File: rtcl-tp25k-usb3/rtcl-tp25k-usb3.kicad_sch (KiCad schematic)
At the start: 65 parts, among them J1 ZX360D-B-10P(30), J10 SSQ-106-02-F-D-RA, J2 0525592253, J3 BTB-DF40C-60DS-0.4V(51), J4 DF40C-60DS-0.4V(51), J5 JTAG, U1 FT601Q, U2 TPD4E05U06DQA, U3 USBLC6-2P6, U4 TPS62826DMQR, X1 ABM3-30.000MHZ-D2Y-T

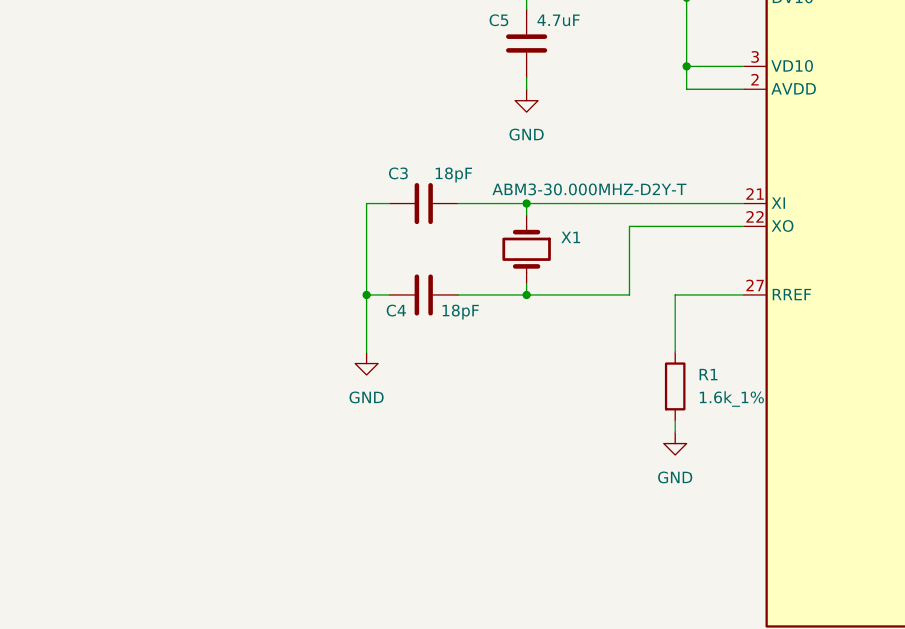
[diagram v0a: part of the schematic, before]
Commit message: WIP
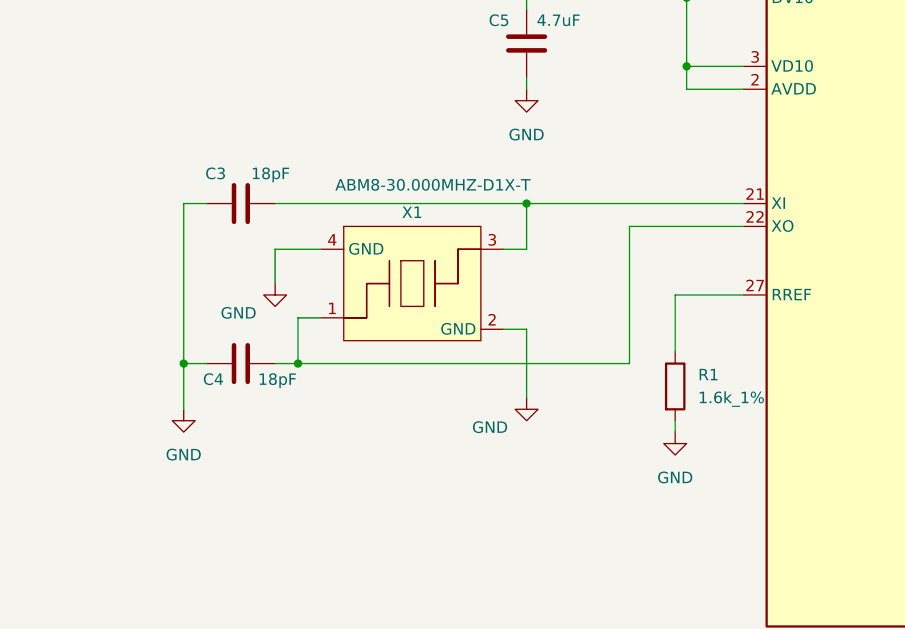
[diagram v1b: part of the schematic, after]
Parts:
- removed X1: ABM3-30.000MHZ-D2Y-T, symbol Device:Crystal
- added X1: ABM8-30.000MHZ-D1X-T, rtcl-p25k-usb3:XTAL_ABM8-30.000MHz-D1X-T, symbol rtcl-tp25k-usb3:ABM8-30.000MHZ-D1X-T
- R52, R53, R54: footprint Resistor_SMD:R_0402_1005Metric -> Resistor_SMD:R_0603_1608Metric_Pad0.98x0.95mm_HandSolder
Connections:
- net GND: now also X1.2 (GND), X1.4 (GND)
- net at C3.2, U1.21 (XI): now also X1.3
- net at C4.2, U1.22 (XO): now also X1.1
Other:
- moved on the sheet: C3, C4

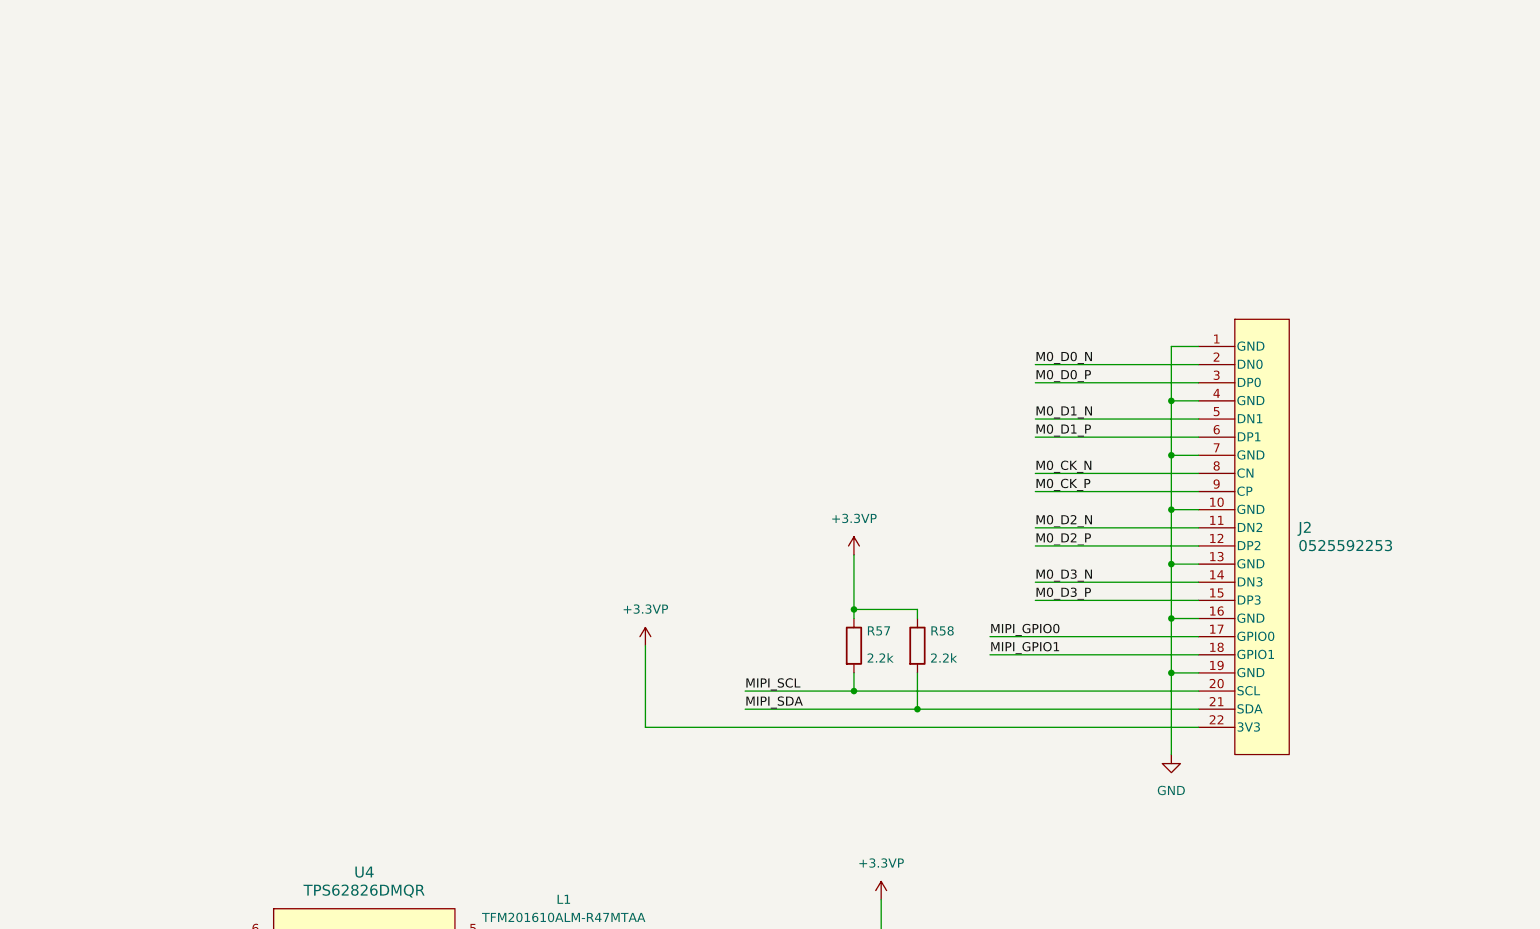
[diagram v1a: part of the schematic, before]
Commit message: WIP
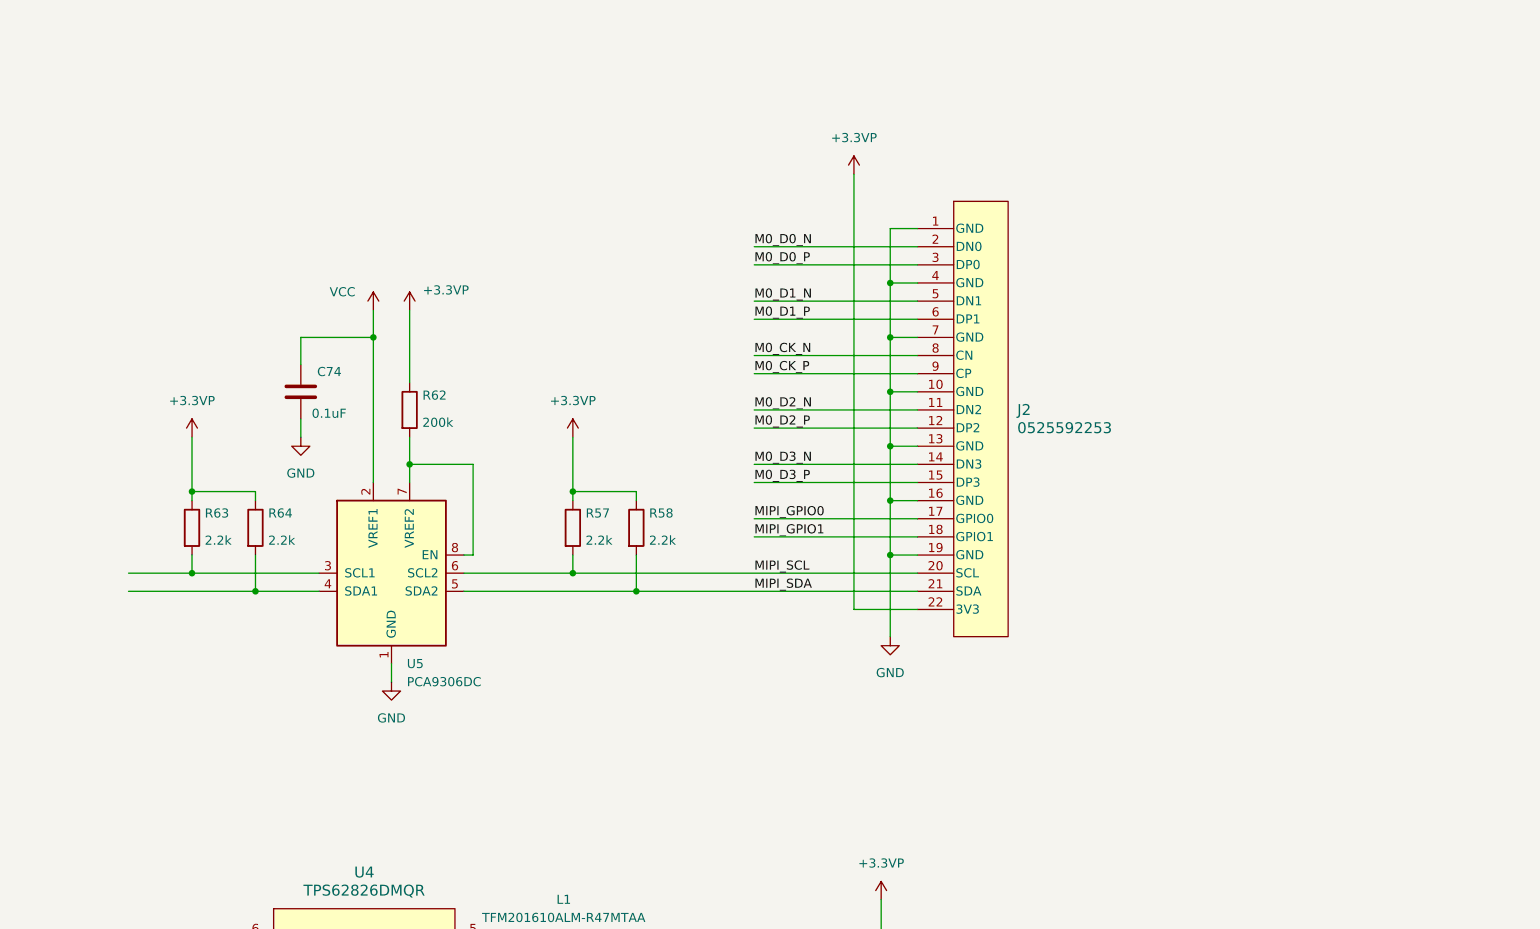
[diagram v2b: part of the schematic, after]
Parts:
- added C74: 0.1uF, Capacitor_SMD:C_0402_1005Metric, symbol Device:C
- added R62: 200k, Resistor_SMD:R_0402_1005Metric, symbol Device:R
- added R63, R64: 2.2k, Resistor_SMD:R_0402_1005Metric, symbol Device:R
- added U5: PCA9306DC, Package_SO:VSSOP-8_2.3x2mm_P0.5mm, symbol Interface:PCA9306DC
- C73: footprint Capacitor_SMD:C_0603_1608Metric -> Capacitor_SMD:C_0402_1005Metric
- C77: footprint Capacitor_SMD:C_0402_1005Metric -> Capacitor_SMD:C_0603_1608Metric
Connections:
- net +3.3VP: now also R62.1, R63.1, R64.1
- net GND: now also C74.2, U5.1 (GND)
- net MIPI_SCL: now also U5.6 (SCL2)
- net MIPI_SDA: now also U5.5 (SDA2)
- net VCC: now also C74.1, U5.2 (VREF1)
- new net: R62.2, U5.7 (VREF2), U5.8 (EN)
- new net: R63.2, U5.3 (SCL1)
- new net: R64.2, U5.4 (SDA1)
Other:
- moved on the sheet: J2, R57, R58
